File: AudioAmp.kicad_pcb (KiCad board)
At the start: 2 copper layers, 134 x 38 mm, 56 parts, among them J1 ACJS-MHOM, J2 ACJS-MHOM, Q1 MJE182G, Q12 MMBT5401, Q13 MMBT5401, Q2 MJE172G, Q3 MMBT5551(RANGE:200-300), Q9 MMBT5551(RANGE:200-300)

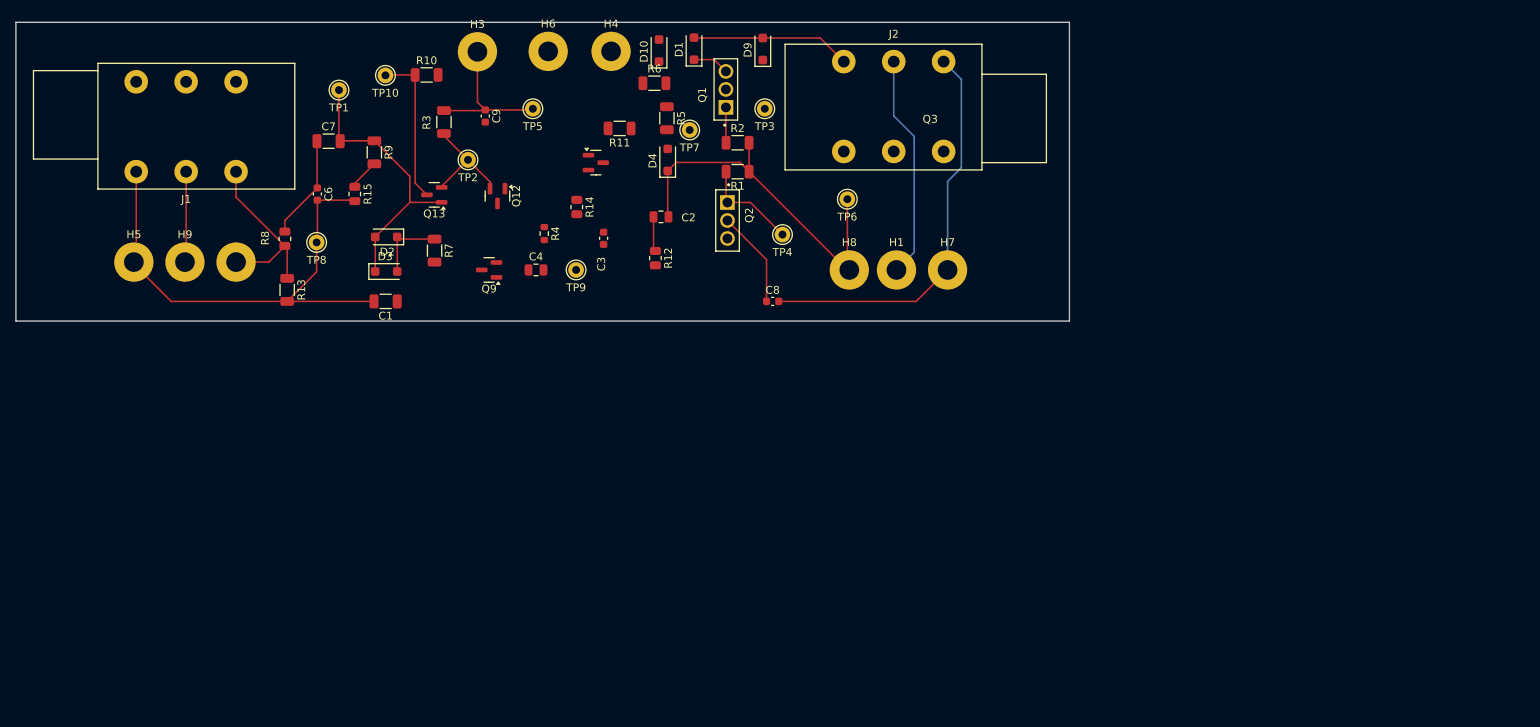
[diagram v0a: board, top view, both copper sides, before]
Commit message: PCB fertig gemacht.
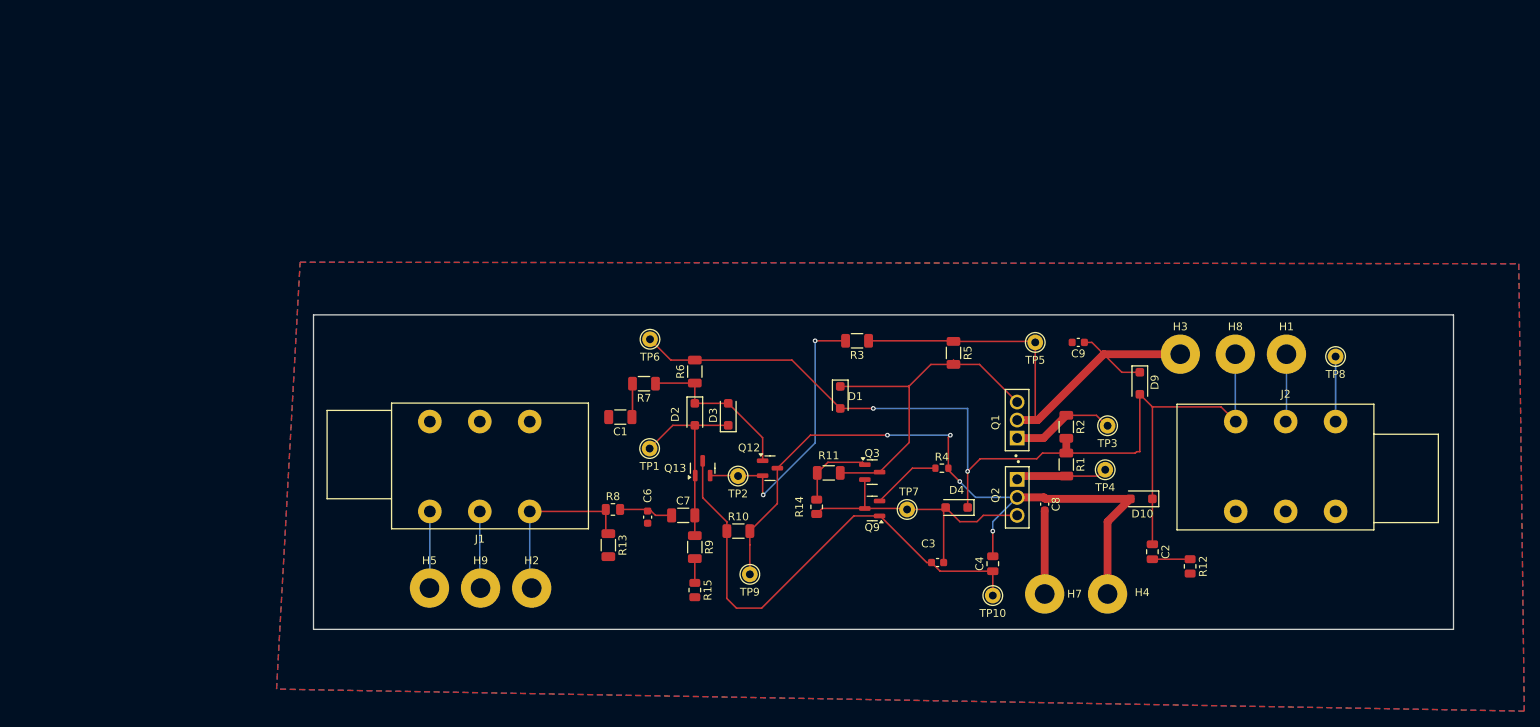
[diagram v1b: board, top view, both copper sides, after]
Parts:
- removed H6: VCC _GND, MountingHole:MountingHole_2.5mm_Pad
- moved TP8 130.4 mm to (195.0, 92.8)
- moved TP10 101.7 mm to (151.4, 123.2)
- moved H3 97.3 mm to (175.2, 92.5)
- moved H4 93.5 mm to (166.0, 123.0)
- moved D10 83.8 mm to (170.3, 110.9), turned to 180 degrees
- moved C9 80.7 mm to (162.3, 91.0), turned to 180 degrees
- moved R12 78.5 mm to (176.5, 119.5)
- moved C2 75.6 mm to (171.7, 117.6), turned to -90 degrees
- moved TP5 70.5 mm to (156.8, 91.0)
- moved R10 70.3 mm to (119.0, 115.0)
- moved C4 69.1 mm to (151.4, 119.2), turned to 90 degrees
- moved J2 67.7 mm to (182.3, 101.1)
- moved R15 66.4 mm to (113.5, 122.5)
- moved C7 65.6 mm to (112.0, 113.0)
- moved R9 64.7 mm to (113.5, 117.0)
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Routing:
- net Net-(C1-Pad2): track 115.0 -> 28.7 mm
- net Net-(D10-A): track 12.4 -> 90.3 mm, vias 0 -> 4
- net Net-(D1-A): track 68.2 -> 128.5 mm, vias 0 -> 2
- net Net-(D9-K): track 19.2 -> 64.2 mm
- net Net-(Q13-C): track 19.7 -> 64.0 mm
- net Net-(D1-K): track 4.68 -> 43.8 mm
- net Net-(D4-A): track 0.00 -> 37.4 mm
- net Net-(Q12-E): track 14.3 -> 35.5 mm, vias 0 -> 2
- net Net-(H1-Pad1): track 28.5 -> 8.61 mm
- net Net-(D2-K): track 9.26 -> 21.0 mm
- net Net-(Q3-B): track 0.00 -> 10.2 mm
- net Net-(D2-A): track 35.3 -> 25.3 mm
- net Net-(Q9-E): track 0.00 -> 8.83 mm
- net Net-(Q1-E): track 4.50 -> 13.2 mm
- net Net-(C6-Pad1): track 13.2 -> 6.86 mm
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- added copper zone on B.Cu, net Net-(C1-Pad2)
- added copper zone on F.Cu, net Net-(C1-Pad2)
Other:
- board size 134 x 38 mm -> 145 x 40 mm
